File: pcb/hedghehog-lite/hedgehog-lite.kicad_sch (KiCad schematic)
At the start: 33 parts, among them J1 Conn_01x04, J2 AVR-ISP-6, SW1 Reset, SW2 SSSS811101, U1 ATmega32U4-M, Y1 16MHz

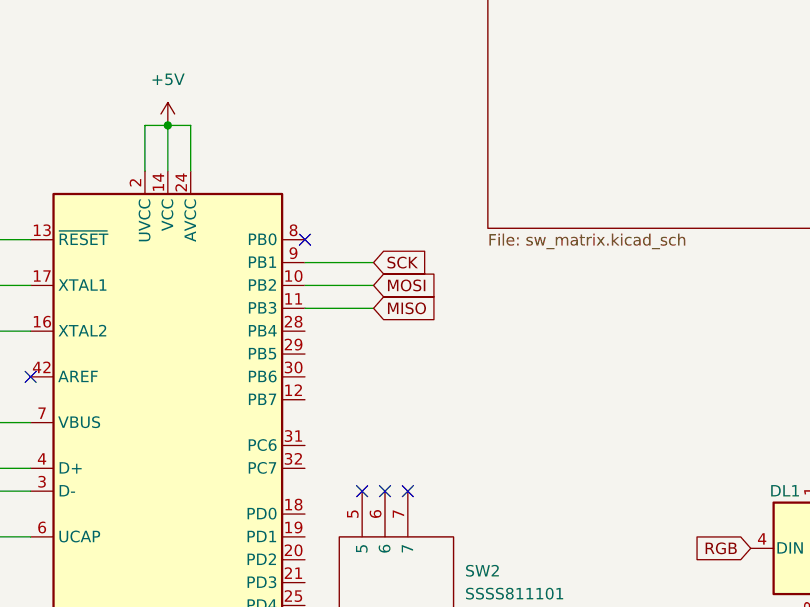
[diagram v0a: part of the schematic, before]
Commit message: Top Row done
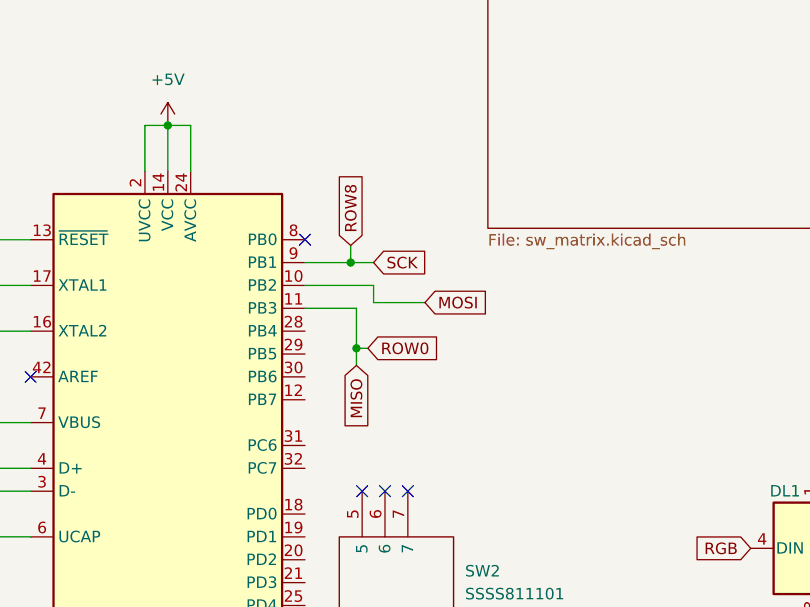
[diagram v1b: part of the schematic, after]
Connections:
- net SCK renamed ROW8
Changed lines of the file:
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@@
   (junction (at 210.82 128.27) (diameter 0) (color 0 0 0 0)
   )
+  (junction (at 97.79 88.9) (diameter 0) (color 0 0 0 0)
+  )
   (junction (at 210.82 113.03) (diameter 0) (color 0 0 0 0)
   )
@@
   )
   (junction (at 74.93 172.72) (diameter 0) (color 0 0 0 0)
+  )
+  (junction (at 98.425 98.425) (diameter 0) (color 0 0 0 0)
   )
   (junction (at 149.86 130.81) (diameter 0) (color 0 0 0 0)
@@
     (stroke (width 0) (type default) (color 0 0 0 0))
   )
+  (wire (pts (xy 98.425 98.425) (xy 99.695 98.425))
+    (stroke (width 0) (type default) (color 0 0 0 0))
+  )
   (wire (pts (xy 195.58 128.27) (xy 210.82 128.27))
     (stroke (width 0) (type default) (color 0 0 0 0))
@@
     (stroke (width 0) (type default) (color 0 0 0 0))
   )
+  (wire (pts (xy 97.79 86.995) (xy 97.79 88.9))
+    (stroke (width 0) (type default) (color 0 0 0 0))
+  )
   (wire (pts (xy 226.06 128.27) (xy 241.3 128.27))
     (stroke (width 0) (type default) (color 0 0 0 0))
@@
     (stroke (width 0) (type default) (color 0 0 0 0))
   )
+  (wire (pts (xy 98.425 98.425) (xy 98.425 100.33))
+    (stroke (width 0) (type default) (color 0 0 0 0))
+  )
   (wire (pts (xy 77.47 73.66) (xy 77.47 78.74))
     (stroke (width 0) (type default) (color 0 0 0 0))
   )
+  (wire (pts (xy 98.425 93.98) (xy 98.425 98.425))
+    (stroke (width 0) (type default) (color 0 0 0 0))
+  )
   (wire (pts (xy 43.18 105.41) (xy 43.18 106.68))
     (stroke (width 0) (type default) (color 0 0 0 0))
@@
     (stroke (width 0) (type default) (color 0 0 0 0))
   )
-  (wire (pts (xy 92.71 88.9) (xy 100.33 88.9))
+  (wire (pts (xy 106.045 93.345) (xy 100.33 93.345))
+    (stroke (width 0) (type default) (color 0 0 0 0))
+  )
+  (wire (pts (xy 92.71 88.9) (xy 97.79 88.9))
     (stroke (width 0) (type default) (color 0 0 0 0))
   )
@@
     (stroke (width 0) (type default) (color 0 0 0 0))
   )
+  (wire (pts (xy 97.79 88.9) (xy 100.33 88.9))
+    (stroke (width 0) (type default) (color 0 0 0 0))
+  )
   (wire (pts (xy 187.96 113.03) (xy 195.58 113.03))
     (stroke (width 0) (type default) (color 0 0 0 0))
@@
     (stroke (width 0) (type default) (color 0 0 0 0))
   )
-  (wire (pts (xy 92.71 93.98) (xy 100.33 93.98))
-    (stroke (width 0) (type default) (color 0 0 0 0))
-  )
   (wire (pts (xy 180.34 113.03) (xy 187.96 113.03))
     (stroke (width 0) (type default) (color 0 0 0 0))
@@
     (stroke (width 0) (type default) (color 0 0 0 0))
   )
+  (wire (pts (xy 100.33 93.345) (xy 100.33 91.44))
+    (stroke (width 0) (type default) (color 0 0 0 0))
+  )
   (wire (pts (xy 48.26 96.52) (xy 62.23 96.52))
     (stroke (width 0) (type default) (color 0 0 0 0))
@@
   )
   (wire (pts (xy 138.43 26.67) (xy 142.24 26.67))
+    (stroke (width 0) (type default) (color 0 0 0 0))
+  )
+  (wire (pts (xy 92.71 93.98) (xy 98.425 93.98))
     (stroke (width 0) (type default) (color 0 0 0 0))
   )
@@
     )
   )
-  (global_label "MOSI" (shape input) (at 100.33 91.44 0) (fields_autoplaced)
-    (effects (font (size 1.27 1.27)) (justify left))
-    (property "Intersheet References" "${INTERSHEET_REFS}" (id 0) (at 19.05 -6.35 0)
+  (global_label "MOSI" (shape input) (at 106.045 93.345 0) (fields_autoplaced)
+    (effects (font (size 1.27 1.27)) (justify left))
+    (property "Intersheet References" "${INTERSHEET_REFS}" (id 0) (at 24.765 -4.445 0)
       (effects (font (size 1.27 1.27)) hide)
     )
@@
     )
   )
-  (global_label "MISO" (shape input) (at 100.33 93.98 0) (fields_autoplaced)
-    (effects (font (size 1.27 1.27)) (justify left))
-    (property "Intersheet References" "${INTERSHEET_REFS}" (id 0) (at 19.05 -6.35 0)
+  (global_label "MISO" (shape input) (at 98.425 100.33 270) (fields_autoplaced)
+    (effects (font (size 1.27 1.27)) (justify right))
+    (property "Intersheet References" "${INTERSHEET_REFS}" (id 0) (at 198.755 19.05 0)
       (effects (font (size 1.27 1.27)) hide)
     )
@@
     )
   )
+  (global_label "ROW8" (shape input) (at 97.79 86.995 90) (fields_autoplaced)
+    (effects (font (size 1.27 1.27)) (justify left))
+    (property "Intersheet References" "${INTERSHEET_REFS}" (id 0) (at 97.7106 79.3205 90)
+      (effects (font (size 1.27 1.27)) (justify left) hide)
+    )
+  )
   (global_label "SCK" (shape input) (at 203.2 34.29 0) (fields_autoplaced)
     (effects (font (size 1.27 1.27)) (justify left))
@@
     )
   )
+  (global_label "ROW0" (shape input) (at 99.695 98.425 0) (fields_autoplaced)
+    (effects (font (size 1.27 1.27)) (justify left))
+    (property "Intersheet References" "${INTERSHEET_REFS}" (id 0) (at 107.3695 98.3456 0)
+      (effects (font (size 1.27 1.27)) (justify left) hide)
+    )
+  )

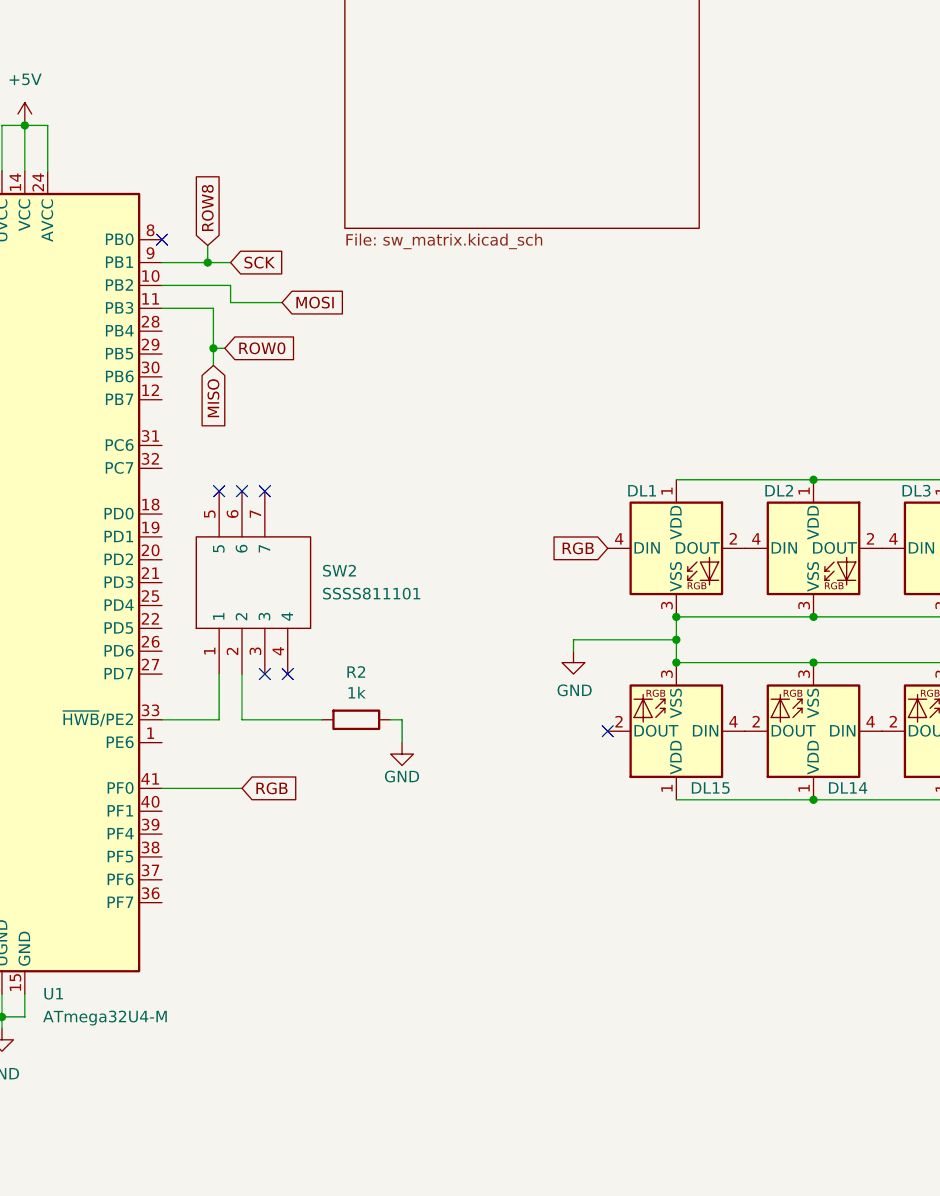
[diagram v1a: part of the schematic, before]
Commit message: All routing done
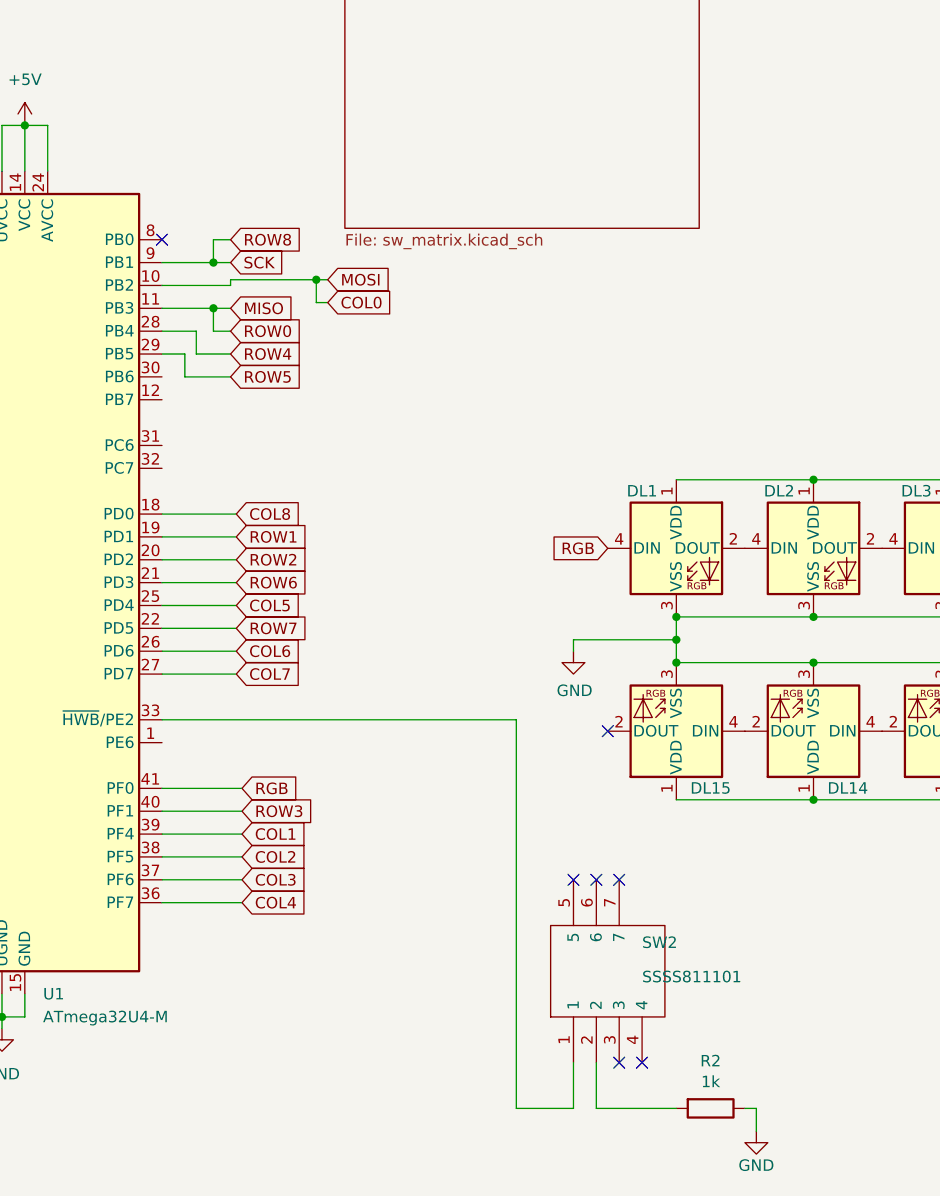
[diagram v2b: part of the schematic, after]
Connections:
- net COL8: now reaches U1.18 (PD0)
- net ROW1: now reaches U1.19 (PD1)
- net ROW2: now reaches U1.20 (PD2)
- net ROW6: now reaches U1.21 (PD3)
- net ROW7: now reaches U1.22 (PD5)
- net COL5: now reaches U1.25 (PD4)
- net COL6: now reaches U1.26 (PD6)
- net COL7: now reaches U1.27 (PD7)
- net ROW4: now reaches U1.28 (PB4)
- net ROW5: now reaches U1.29 (PB5)
- net COL4: now reaches U1.36 (PF7)
- net COL3: now reaches U1.37 (PF6)
- net COL2: now reaches U1.38 (PF5)
- net COL1: now reaches U1.39 (PF4)
- net ROW3: now reaches U1.40 (PF1)
- net MOSI renamed COL0
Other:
- moved on the sheet: R2, SW2
